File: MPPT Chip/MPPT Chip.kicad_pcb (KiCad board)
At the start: 2 copper layers, 2 parts

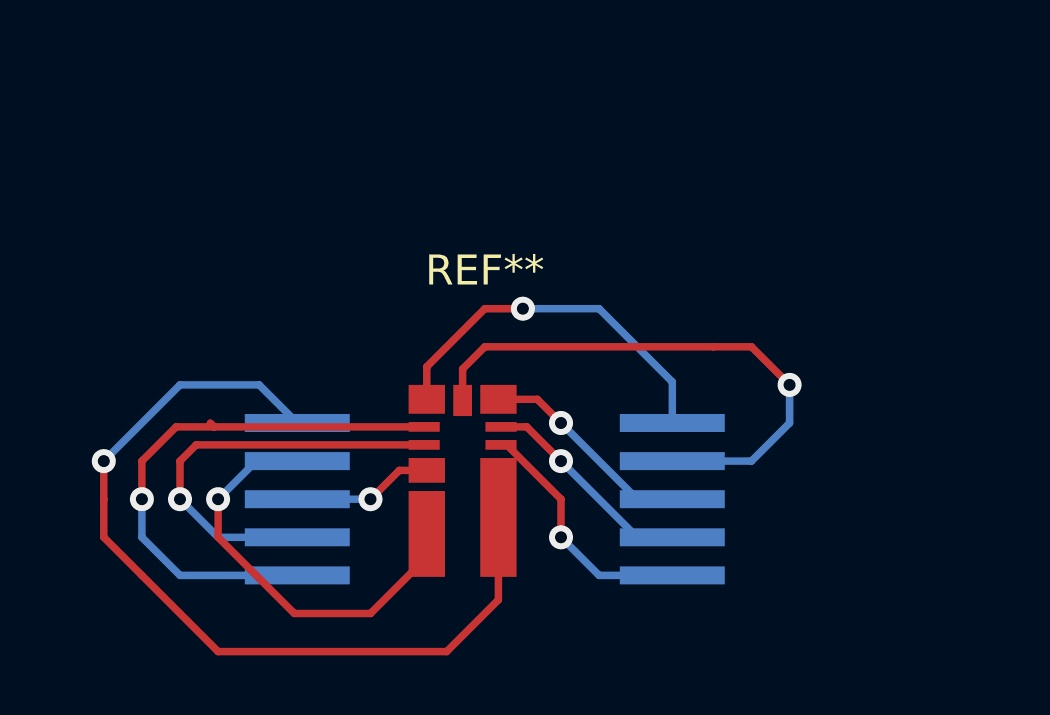
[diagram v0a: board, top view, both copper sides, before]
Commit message: 11/10 meeting updates
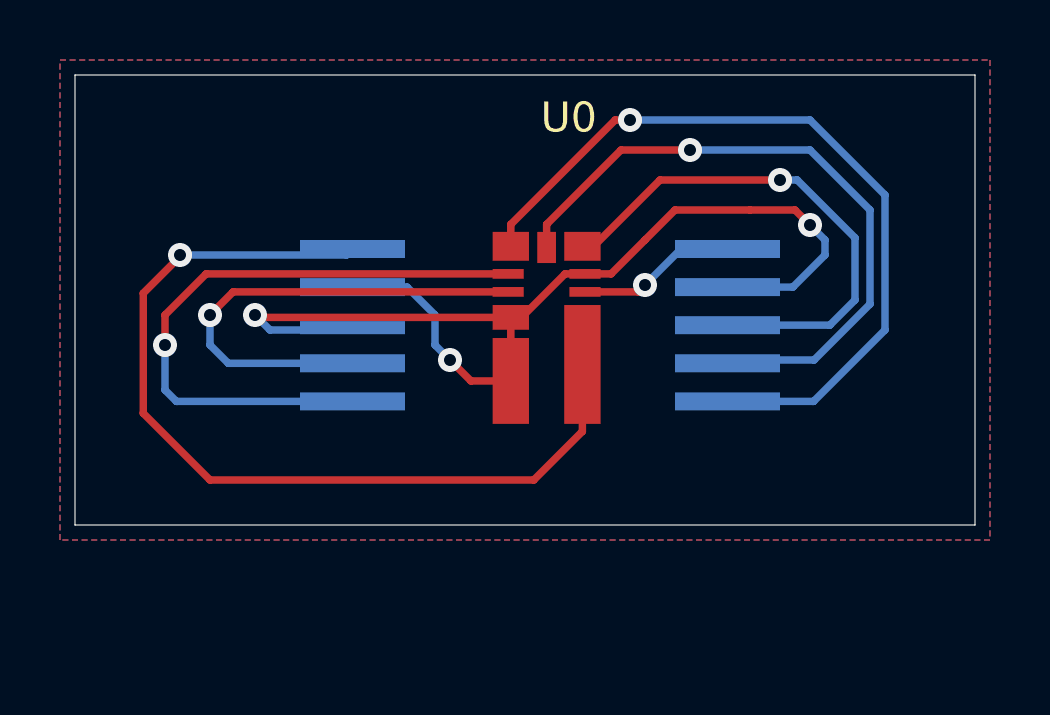
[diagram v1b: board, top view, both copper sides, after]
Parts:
- removed REF**: MAX20801, MAX20801:MAX20801
- removed REF**: PinHeader, MAX20801:PinHeader
- added J1: Conn_02x05_Counter_Clockwise, MAX20801:PinHeader, B.Cu at (75.5, 98.3)
- added U0: MAX20801, MAX20801:MAX20801, F.Cu at (79.0, 96.5)
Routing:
- net (no net): track 132.3 -> 0.00 mm, vias 10 -> 0
- net GND: track 0.00 -> 37.9 mm, vias 0 -> 3
- net Net-(J1-Pad5): track 0.00 -> 30.1 mm, vias 0 -> 1
- net Net-(J1-Pad10): track 0.00 -> 26.4 mm, vias 0 -> 1
- net Net-(J1-Pad9): track 0.00 -> 22.1 mm, vias 0 -> 1
- net Net-(J1-Pad1): track 0.00 -> 20.9 mm, vias 0 -> 1
- net Net-(J1-Pad8): track 0.00 -> 17.5 mm, vias 0 -> 1
- net Net-(J1-Pad2): track 0.00 -> 16.3 mm, vias 0 -> 1
- net Net-(J1-Pad6): track 0.00 -> 5.34 mm, vias 0 -> 1
- added copper zone on B.Cu, net GND
- added copper zone on F.Cu, net GND
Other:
- board outline added: 30 x 15 mm
